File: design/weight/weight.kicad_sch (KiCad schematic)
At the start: 33 parts, among them J2 Conn_01x02_Pin, Q1 2N3904, U1 LM13700, U2 LM324, U3 LM324

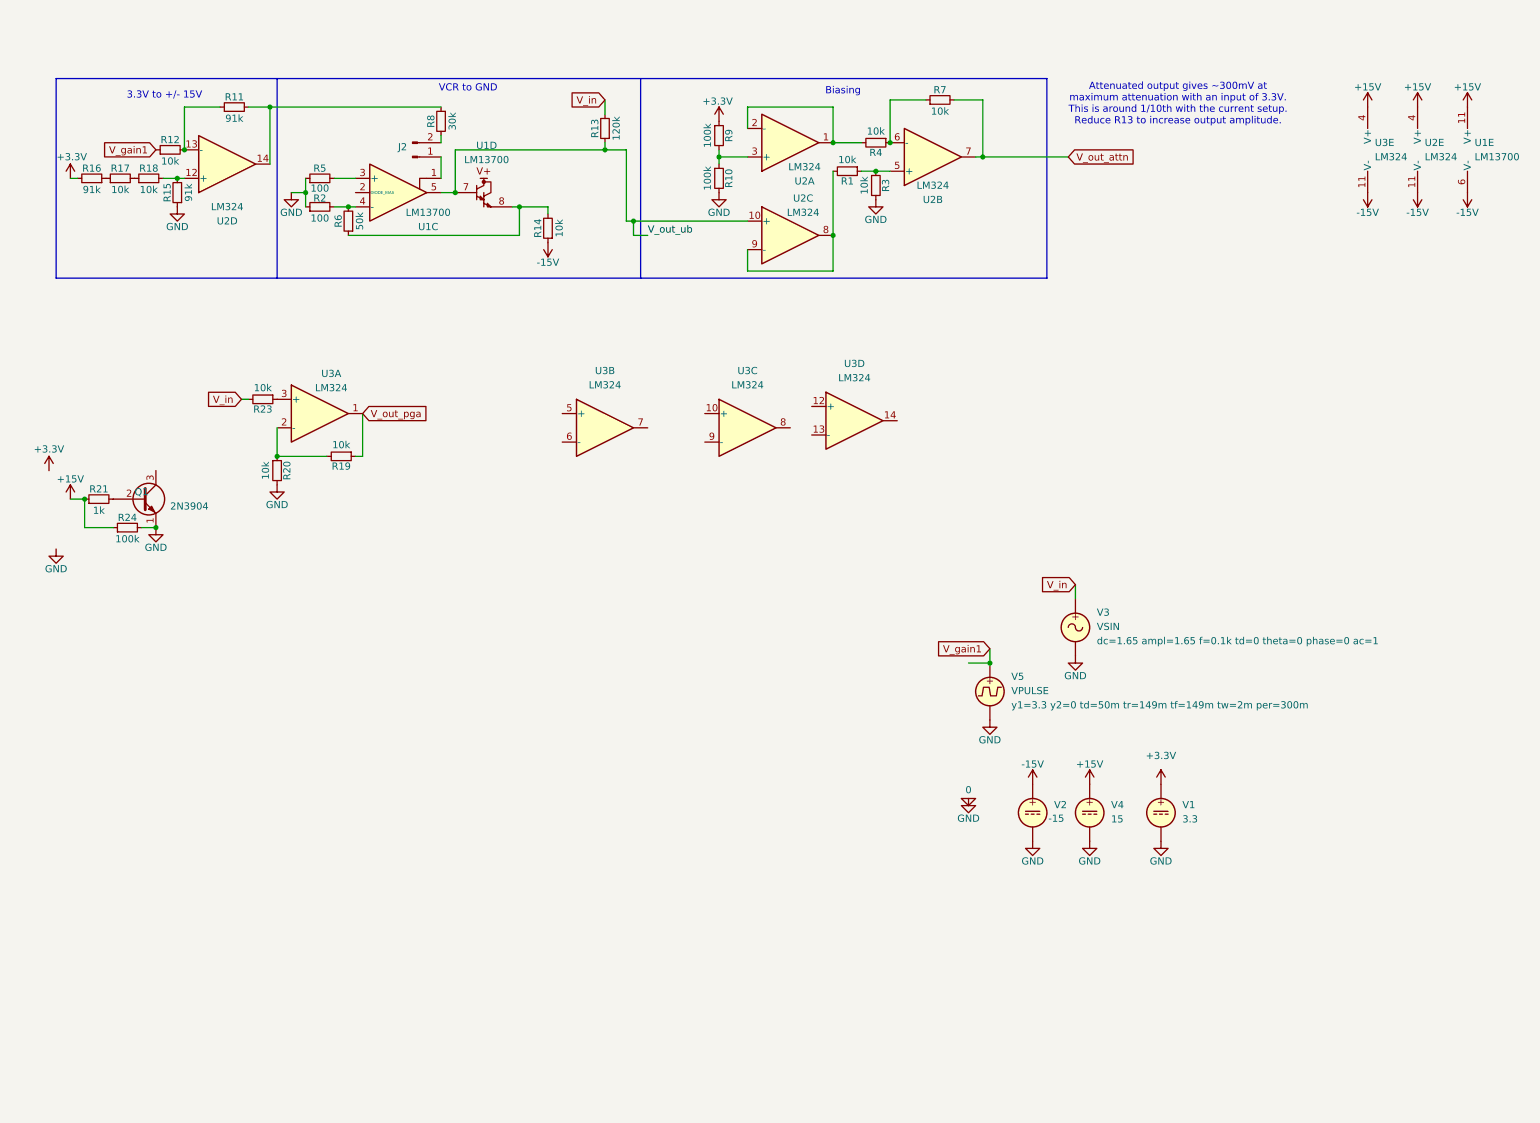
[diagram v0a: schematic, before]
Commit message: Finished the weight design
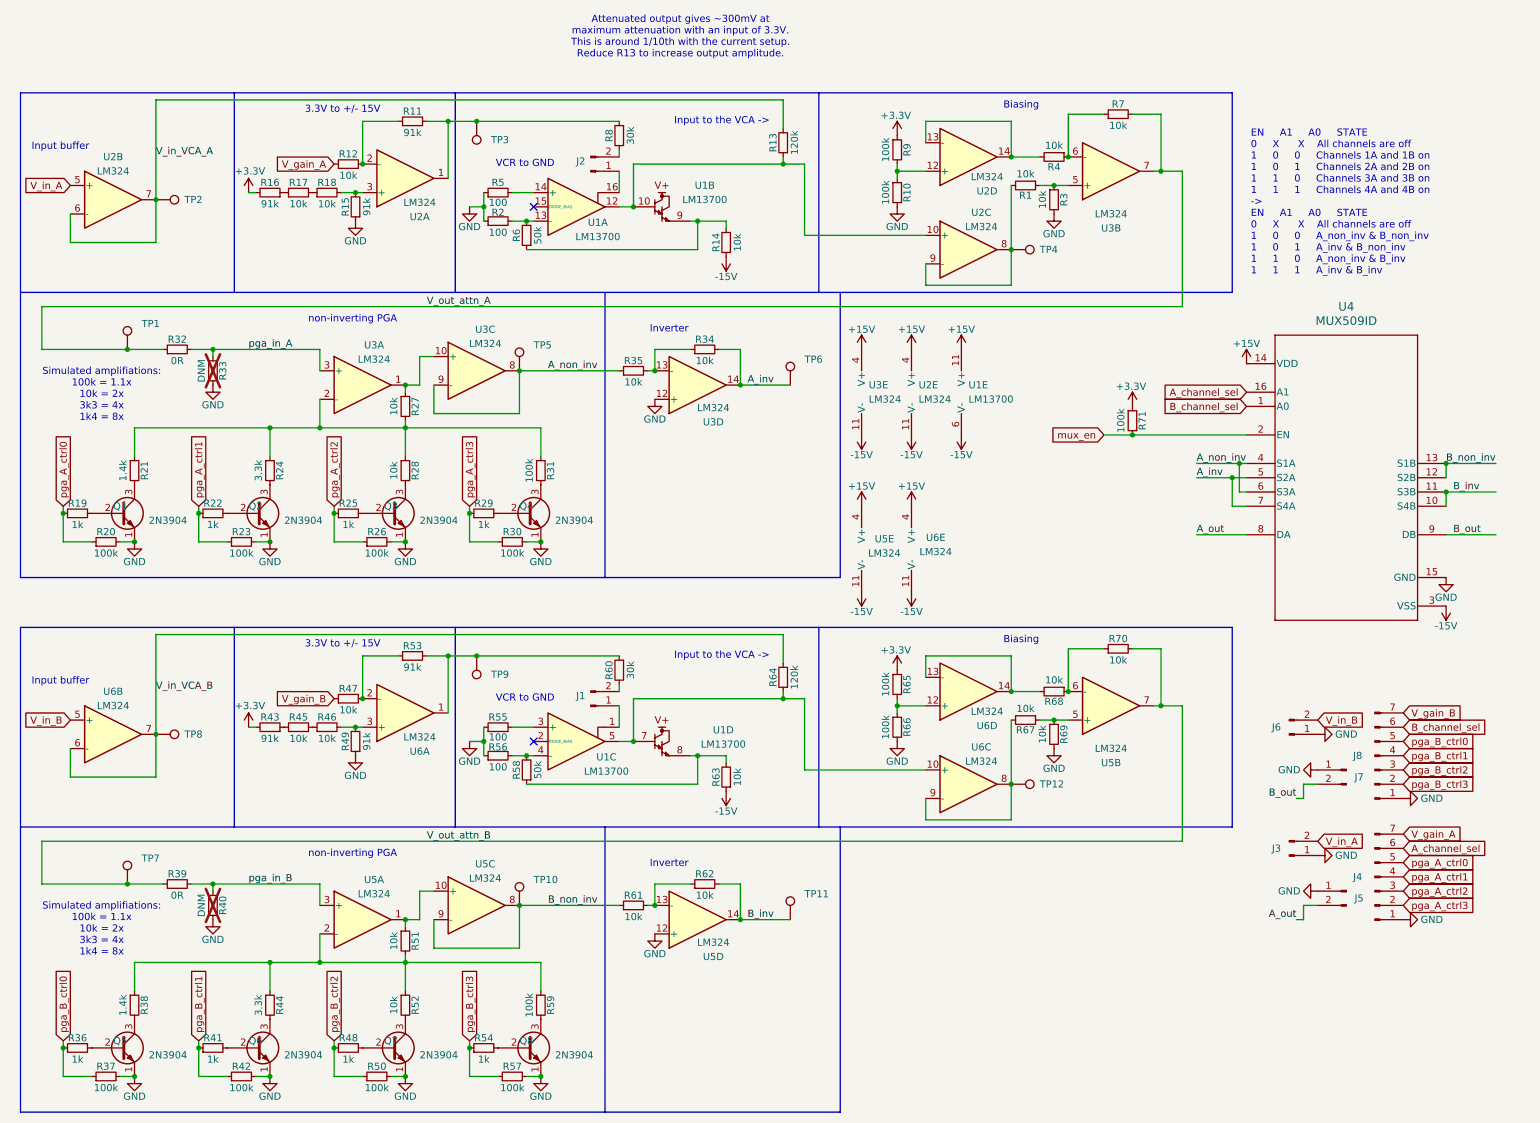
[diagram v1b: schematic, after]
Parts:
- removed V1: 3.3, symbol Simulation_SPICE:VDC
- removed V2: -15, symbol Simulation_SPICE:VDC
- removed V3: VSIN, symbol Simulation_SPICE:VSIN
- removed V4: 15, symbol Simulation_SPICE:VDC
- removed V5: VPULSE, symbol Simulation_SPICE:VPULSE
- added J1, J3, J5, J6, J7: Conn_01x02_Pin, Connector_PinHeader_2.54mm:PinHeader_1x02_P2.54mm_Vertical, symbol Connector:Conn_01x02_Pin
- added J4, J8: Conn_01x07_Pin, Connector_PinHeader_2.54mm:PinHeader_1x07_P2.54mm_Vertical, symbol Connector:Conn_01x07_Pin
- added Q2, Q3, Q4, Q5, Q6, Q7, Q8: 2N3904, Package_TO_SOT_THT:TO-92_Inline, symbol Transistor_BJT:2N3904
- added R22, R25, R29, R36, R41, R48, R54: 1k, Resistor_SMD:R_0402_1005Metric, symbol Device:R_Small
- added R26, R30, R31, R37, R42, R50, R57, R59, R65, R66, R71: 100k, Resistor_SMD:R_0402_1005Metric, symbol Device:R_Small
- added R27, R28, R34, R35, R45, R46, R47, R51, R52, R61, R62, R63, R67, R68, R69, R70: 10k, Resistor_SMD:R_0402_1005Metric, symbol Device:R_Small
- added R32, R39: 0R, Resistor_SMD:R_0402_1005Metric, symbol Device:R_Small
- added R33, R40: DNM, Resistor_SMD:R_0402_1005Metric, symbol Device:R_Small
- added R38: 1.4k, Resistor_SMD:R_0402_1005Metric, symbol Device:R_Small
- added R43, R49, R53: 91k, Resistor_SMD:R_0402_1005Metric, symbol Device:R_Small
- added R44: 3.3k, Resistor_SMD:R_0402_1005Metric, symbol Device:R_Small
- added R55, R56: 100, Resistor_SMD:R_0402_1005Metric, symbol Device:R_Small
- added R58: 50k, Resistor_SMD:R_0402_1005Metric, symbol Device:R_Small
- added R60: 30k, Resistor_SMD:R_0402_1005Metric, symbol Device:R_Small
- added R64: 120k, Resistor_SMD:R_0402_1005Metric, symbol Device:R_Small
- added TP1, TP10, TP11, TP12, TP2, TP3, TP4, TP5, TP6, TP7, TP8, TP9: TestPoint, Connector_PinHeader_2.54mm:PinHeader_1x01_P2.54mm_Vertical, symbol Connector:TestPoint
- added unit 1 of U1
- added unit 2 of U1
- added U4: MUX509ID, footprints:D0016A_N, symbol MUX509ID:MUX509ID
- added U5, U6: LM324, LM324:SOIC127P600X175-14N, symbol Amplifier_Operational:LM324
- R19: value 10k -> 1k
- R20, R23: value 10k -> 100k
- R21: value 1k -> 1.4k
- R24: value 100k -> 3.3k
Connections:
- net +15V: now also U4.14 (VDD), U5.4 (V+), U6.4 (V+); no longer R21.1, R24.1
- net +3.3V: now also R43.2, R65.1, R71.1
- net -15V: now also R63.1, U4.3 (VSS), U5.11 (V-), U6.11 (V-)
- net pga_A_ctrl1: now reaches R23.1
- net pga_A_ctrl1: now also J4.4 (Pin_4), R22.1; no longer U3.3 (+)
- net at R5.2: now also U1.14 (+); no longer U1.3 (+)
- net at U3.5 (+): now also R1.1, R3.1
- net at U3.6 (-): now also R4.1, R7.1
- net V_out_attn_A: now reaches U3.7
- net V_out_attn_A: now also R7.2, R32.1, TP1.1
- net at J2.1 (Pin_1): now also U1.16; no longer U1.1
- net at R15.2, R18.2: now also U2.3 (+); no longer U2.12 (+)
- net at R1.2, U2.8, U2.9 (-): now also TP4.1
- net at R10.1, R9.2: now also U2.12 (+); no longer U2.3 (+)
- net at R2.2, R6.2: now also U1.13 (-); no longer U1.4 (-)
- net at R14.2, R6.1: now also U1.9; no longer U1.8
- net at R11.2, R8.1: now also U2.1, TP3.1; no longer U2.14
- net at R21.2: now also Q1.3 (C); no longer Q1.2 (B)
- net at R11.1, R12.2: now also U2.2 (-); no longer U2.13 (-)
- net GND: now reaches U3.12 (+)
- net GND: now also Q1.1 (E), R10.2, R15.1, R2.1, R20.2, R23.2, R3.2, R5.1, J3.1 (Pin_1), J4.1 (Pin_1), J5.1 (Pin_1), J6.1 (Pin_1), J7.1 (Pin_1), J8.1 (Pin_1), Q2.1 (E), Q3.1 (E), Q4.1 (E), Q5.1 (E), Q6.1 (E), Q7.1 (E), Q8.1 (E), R26.2, R30.2, R33.2, R37.2, R40.2, R42.2, R49.1, R50.2, R55.1, R56.1, R57.2, R66.2, R69.2, U4.15 (GND), U5.12 (+)
- net at U3.13 (-): now also R34.1, R35.2
- net A_inv: now reaches U3.14
- net A_inv: now also R34.2, TP6.1, U4.5 (S2A), U4.7 (S4A)
- net at U3.10 (+): now also U3.1, R27.1
- net A_non_inv: now reaches U3.8
- net A_non_inv: now also U3.9 (-), R35.1, TP5.1, U4.4 (S1A), U4.6 (S3A)
- removed net 0: Q1.1 (E), R10.2, R15.1, R2.1, R20.2, R24.2, R3.2, R5.1
- net V_gain1 renamed V_gain_A
- net V_gain_A: now also J4.7 (Pin_7)
- net V_in renamed V_in_VCA_A
- net V_in_VCA_A: now also U2.6 (-), U2.7, TP2.1; no longer R23.2
- removed net V_out_attn: R7.2, U2.7
- net V_out_pga renamed pga_A_ctrl0
- net pga_A_ctrl0: now also R20.1, J4.5 (Pin_5); no longer U3.1
- net V_out_ub: no longer names the net of U1.5, U1.7
- net V_out_ub: now also R64.1, U6.10 (+); no longer R13.1, U2.10 (+)
- new net: R58.1, R63.2, U1.8
- new net: Q8.2 (B), R54.2
- new net: Q8.3 (C), R59.2
- new net: R13.1, U1.10, U1.12, U2.10 (+)
- new net: R21.1, R24.1, R27.2, R28.1, R31.1, U3.2 (-)
- new net: R51.1, U5.1, U5.10 (+)
- new net: R38.1, R44.1, R51.2, R52.1, R59.1, U5.2 (-)
- new net: R55.2, U1.3 (+)
- new net: R61.2, R62.1, U5.13 (-)
- new net: R47.2, R53.1, U6.2 (-)
- new net: Q4.3 (C), R31.2
- new net: Q3.3 (C), R28.2
- new net: R68.1, R70.1, U5.6 (-)
- new net: R68.2, U6.13 (-), U6.14
- new net: R65.2, R66.1, U6.12 (+)
- new net: R56.2, R58.2, U1.4 (-)
- new net: R4.2, U2.13 (-), U2.14
- new net: Q6.2 (B), R41.2
- new net: Q5.3 (C), R38.2
- new net: Q5.2 (B), R36.2
- new net: Q6.3 (C), R44.2
- new net: R45.2, R46.1
- new net: R46.2, R49.2, U6.3 (+)
- new net: R53.2, R60.1, TP9.1, U6.1
- new net: J1.2 (Pin_2), R60.2
- new net: Q7.3 (C), R52.2
- new net: R67.2, TP12.1, U6.8, U6.9 (-)
- new net: R67.1, R69.1, U5.5 (+)
- new net: R43.1, R45.1
- new net: Q7.2 (B), R48.2
- new net: Q4.2 (B), R29.2
- new net: Q2.2 (B), R22.2
- new net: Q2.3 (C), R24.2
- new net: Q1.2 (B), R19.2
- new net: Q3.2 (B), R25.2
- new net: J1.1 (Pin_1), U1.1
- new net A_channel_sel: J4.6 (Pin_6), U4.16 (A1)
- new net A_out: J5.2 (Pin_2), U4.8 (DA)
- new net B_channel_sel: J8.6 (Pin_6), U4.1 (A0)
- new net B_inv: R62.2, TP11.1, U4.10 (S4B), U4.11 (S3B), U5.14
- new net B_non_inv: R61.1, TP10.1, U4.12 (S2B), U4.13 (S1B), U5.8, U5.9 (-)
- new net B_out: J7.2 (Pin_2), U4.9 (DB)
- new net V_gain_B: J8.7 (Pin_7), R47.1
- new net V_in_A: J3.2 (Pin_2), U2.5 (+)
- new net V_in_B: J6.2 (Pin_2), U6.5 (+)
- new net V_in_VCA_B: R64.2, TP8.1, U6.6 (-), U6.7
- new net V_out_attn_B: R39.1, R70.2, TP7.1, U5.7
- new net mux_en: R71.2, U4.2 (EN)
- new net pga_A_ctrl2: J4.3 (Pin_3), R25.1, R26.1
- new net pga_A_ctrl3: J4.2 (Pin_2), R29.1, R30.1
- new net pga_B_ctrl0: J8.5 (Pin_5), R36.1, R37.1
- new net pga_B_ctrl1: J8.4 (Pin_4), R41.1, R42.1
- new net pga_B_ctrl2: J8.3 (Pin_3), R48.1, R50.1
- new net pga_B_ctrl3: J8.2 (Pin_2), R54.1, R57.1
- new net pga_in_A: R32.2, R33.1, U3.3 (+)
- new net pga_in_B: R39.2, R40.1, U5.3 (+)
- no-connect marks 0 -> 2
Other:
- note added: "EN A1 A0 STATE 0 X X All channels are off 1 0 0 Channels 1A and 1B on 1 0 1 Channels 2A and 2B on 1 1 0 Channels 3A and 3B on 1 1 1 Channels 4A and 4B on -> EN A1 A0 STATE 0 X X All channels are off 1 0 0 A_non_inv & B_non_inv 1 0 1 A_inv & B_non_inv 1 1 0 A_non_inv & B_inv 1 1 1 A_inv & B_inv"
- note added: "Input buffer"
- note added: "Input to the VCA ->"
- note added: "Inverter"
- note added: "Simulated amplifiations: 100k = 1.1x 10k = 2x 3k3 = 4x 1k4 = 8x"
- note added: "non-inverting PGA"
- moved on the sheet: J2, R1, R10, R11, R12, R13, R14, R15, R16, R17, R18, R2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
